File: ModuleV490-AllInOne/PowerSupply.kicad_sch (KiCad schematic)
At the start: 28 parts, among them J5 POWER_IN, J9 BYPASS, U10 XL7005A, U11 AP2204K-5.0TRG1, U12 XC6206-1.8NR, U9 XC6206-3.3V

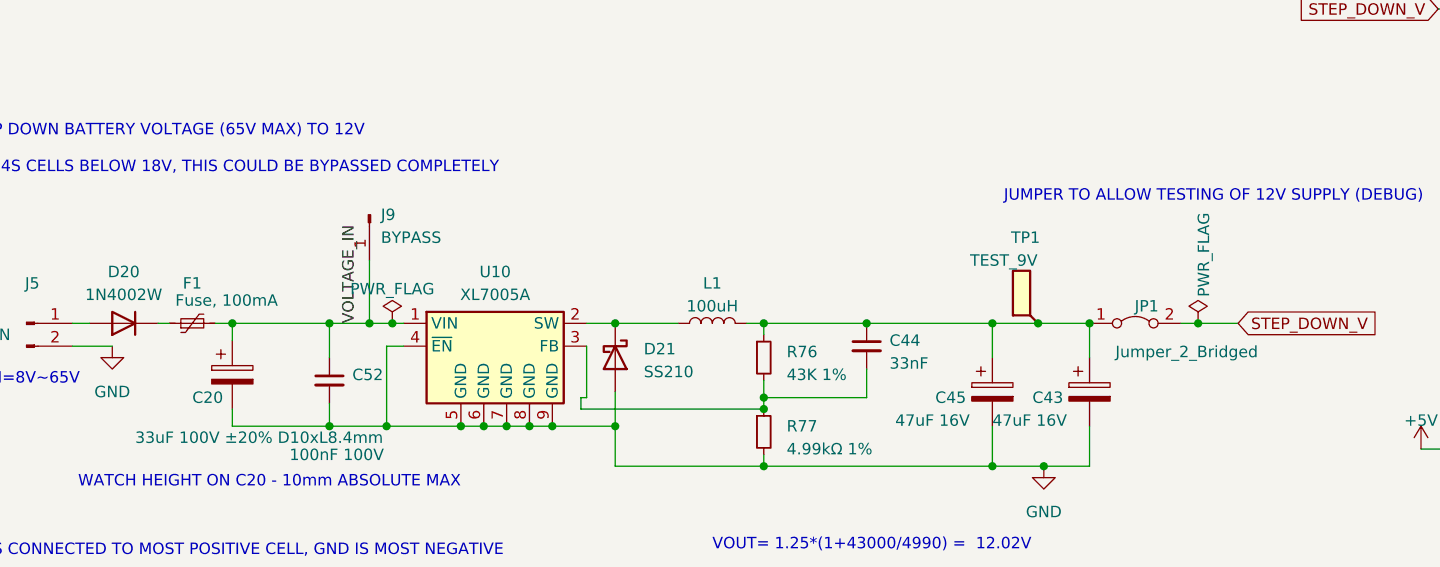
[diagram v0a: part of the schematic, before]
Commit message: Squashed commit of the following:
commit 382df4b7a104fb34cc4a4da3f786b21ade19fcd5
Author: GitHub Action <action@github.com>
Date:   Fri Apr 18 11:47:05 2025 +0000

    CI: pcb-artifacts-ModuleV490-AllInOne

commit b35cb7a0d3894cf57b33edb037eb829bc9ec5ea4
Author: Stuart Pittaway <1201909+stuartpittaway@users.noreply.github.com>
Date:   Fri Apr 18 12:44:57 2025 +0100

    Minor tweaks

commit ea046b7e5d836263693da1b47c6dfb3dc918925c
Author: Stuart Pittaway <1201909+stuartpittaway@users.noreply.github.com>
Date:   Fri Apr 18 12:44:16 2025 +0100

    PCB Panel of Temp sensors

commit ba929f4700586b6858203bc466c6b18e911d661e
Author: GitHub Action <action@github.com>
Date:   Sun Mar 23 15:29:50 2025 +0000

    CI: pcb-artifacts-ModuleV490-AllInOne

commit 1dbbac7378fdc5acb48c43d3f728917ce2318f16
Author: GitHub Action <action@github.com>
Date:   Wed Apr 10 09:57:21 2024 +0000

    CI: pcb-artifacts-ModuleV490-AllInOne

commit 35f617d42fc7a6a7ab395d232005d3307c26595c
Author: Stuart Pittaway <1201909+stuartpittaway@users.noreply.github.com>
Date:   Wed Apr 10 10:55:49 2024 +0100

    Update pcb-artifacts-modulev490-allinone.yaml

commit c8295c0089ea2c5e86742be6a5572142963deb8f
Author: Stuart Pittaway <1201909+stuartpittaway@users.noreply.github.com>
Date:   Wed Apr 10 10:53:50 2024 +0100

    Update pcb-artifacts-modulev490-allinone.yaml

commit d19b2989a6afd4cac4ecf3c8c78554eedba7b99a
Author: Stuart Pittaway <1201909+stuartpittaway@users.noreply.github.com>
Date:   Wed Apr 10 10:50:28 2024 +0100

    Update pcb-artifacts-modulev490-allinone.yaml

commit 8478886fe70d1ee53aca3bbd908099e6f38ff11d
Author: Stuart Pittaway <1201909+stuartpittaway@users.noreply.github.com>
Date:   Wed Apr 10 10:41:28 2024 +0100

    Update pcb-artifacts-modulev490-allinone.yaml

commit afeafa74721a9b51459c6106f0a15ae423229204
Author: Stuart Pittaway <1201909+stuartpittaway@users.noreply.github.com>
Date:   Wed Apr 10 10:39:10 2024 +0100

    Inductor part change - fix workflows

commit 70fd25ba43b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
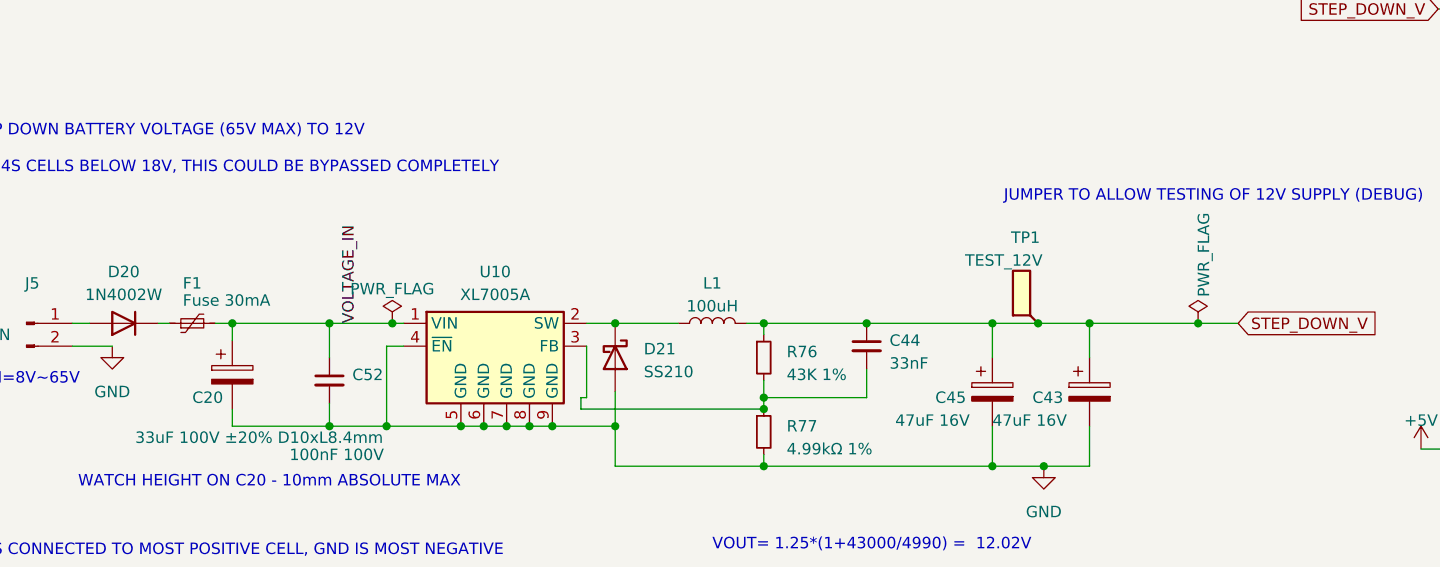
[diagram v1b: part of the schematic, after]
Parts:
- removed J9: BYPASS, Connector_PinSocket_2.54mm:PinSocket_1x01_P2.54mm_Vertical, symbol Connector:Conn_01x01_Pin
- removed JP1: Jumper_2_Bridged, Connector_PinHeader_2.54mm:PinHeader_1x02_P2.54mm_Vertical, symbol Jumper:Jumper_2_Bridged
- F1: value Fuse, 100mA -> Fuse 30mA; footprint Fuse:Fuse_Bourns_MF-RHT100 -> Fuse:Fuse_0805_2012Metric; LCSCStockCode C2680606 -> C19273358; PartNumber JK250-100U -> 0805L003/80XR
- L1: footprint COILMX:MS1040-101M -> Inductor_SMD:L_1008_2520Metric_Pad1.43x2.20mm_HandSolder; LCSCStockCode C380060 -> C286551; PartNumber MS1040-101M -> NLV25T-101J-EF
- TP1: value TEST_9V -> TEST_12V
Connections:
- net STEP_DOWN_V: now also C43.1, C44.1, C45.1, L1.2, R76.1, TP1.1
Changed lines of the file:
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@@
   (junction (at 228.6 121.285) (diameter 0) (color 0 0 0 0)
   )
+  (junction (at 210.185 48.26) (diameter 0) (color 0 0 0 0)
+  )
+  (junction (at 64.135 73.025) (diameter 0) (color 0 0 0 0)
+  )
+  (junction (at 208.28 131.445) (diameter 0) (color 0 0 0 0)
+  )
+  (junction (at 64.135 84.455) (diameter 0) (color 0 0 0 0)
+  )
+  (junction (at 205.105 97.155) (diameter 0) (color 0 0 0 0)
+  )
+  (junction (at 112.395 81.28) (diameter 0) (color 0 0 0 0)
+  )
+  (junction (at 70.485 84.455) (diameter 0) (color 0 0 0 0)
+  )
+  (junction (at 78.74 84.455) (diameter 0) (color 0 0 0 0)
+  )
+  (junction (at 201.295 38.1) (diameter 0) (color 0 0 0 0)
+  )
+  (junction (at 88.9 84.455) (diameter 0) (color 0 0 0 0)
+  )
+  (junction (at 191.135 121.285) (diameter 0) (color 0 0 0 0)
+  )
+  (junction (at 219.71 121.285) (diameter 0) (color 0 0 0 0)
+  )
+  (junction (at 71.12 73.025) (diameter 0) (color 0 0 0 0)
+  )
+  (junction (at 53.34 73.025) (diameter 0) (color 0 0 0 0)
+  )
+  (junction (at 143.51 88.9) (diameter 0) (color 0 0 0 0)
+  )
+  (junction (at 137.795 88.9) (diameter 0) (color 0 0 0 0)
+  )
+  (junction (at 112.395 88.9) (diameter 0) (color 0 0 0 0)
+  )
+  (junction (at 123.825 73.025) (diameter 0) (color 0 0 0 0)
+  )
+  (junction (at 228.6 86.995) (diameter 0) (color 0 0 0 0)
+  )
+  (junction (at 142.875 73.025) (diameter 0) (color 0 0 0 0)
+  )
+  (junction (at 95.885 73.025) (diameter 0) (color 0 0 0 0)
+  )
   (junction (at 148.59 73.025) (diameter 0) (color 0 0 0 0)
   )
-  (junction (at 210.185 48.26) (diameter 0) (color 0 0 0 0)
-  )
-  (junction (at 64.135 73.025) (diameter 0) (color 0 0 0 0)
-  )
-  (junction (at 208.28 131.445) (diameter 0) (color 0 0 0 0)
-  )
-  (junction (at 64.135 84.455) (diameter 0) (color 0 0 0 0)
-  )
-  (junction (at 205.105 97.155) (diameter 0) (color 0 0 0 0)
-  )
-  (junction (at 112.395 81.28) (diameter 0) (color 0 0 0 0)
-  )
-  (junction (at 70.485 84.455) (diameter 0) (color 0 0 0 0)
-  )
-  (junction (at 78.74 84.455) (diameter 0) (color 0 0 0 0)
-  )
-  (junction (at 201.295 38.1) (diameter 0) (color 0 0 0 0)
-  )
-  (junction (at 88.9 84.455) (diameter 0) (color 0 0 0 0)
-  )
-  (junction (at 191.135 121.285) (diameter 0) (color 0 0 0 0)
-  )
-  (junction (at 219.71 121.285) (diameter 0) (color 0 0 0 0)
-  )
-  (junction (at 71.12 73.025) (diameter 0) (color 0 0 0 0)
-  )
-  (junction (at 68.58 73.025) (diameter 0) (color 0 0 0 0)
-  )
-  (junction (at 53.34 73.025) (diameter 0) (color 0 0 0 0)
-  )
-  (junction (at 143.51 88.9) (diameter 0) (color 0 0 0 0)
-  )
-  (junction (at 137.795 88.9) (diameter 0) (color 0 0 0 0)
-  )
-  (junction (at 112.395 88.9) (diameter 0) (color 0 0 0 0)
-  )
-  (junction (at 123.825 73.025) (diameter 0) (color 0 0 0 0)
-  )
-  (junction (at 228.6 86.995) (diameter 0) (color 0 0 0 0)
-  )
-  (junction (at 142.875 73.025) (diameter 0) (color 0 0 0 0)
-  )
-  (junction (at 95.885 73.025) (diameter 0) (color 0 0 0 0)
-  )
   (junction (at 137.795 73.025) (diameter 0) (color 0 0 0 0)
   )
+  (junction (at 160.655 73.025) (diameter 0) (color 0 0 0 0)
+  )
   (junction (at 221.615 38.1) (diameter 0) (color 0 0 0 0)
   )
@@
   (junction (at 112.395 73.025) (diameter 0) (color 0 0 0 0)
   )
-  (junction (at 160.655 73.025) (diameter 0) (color 0 0 0 0)
-  )
   (junction (at 219.71 86.995) (diameter 0) (color 0 0 0 0)
   )
@@
     (stroke (width 0) (type default))
   )
-  (wire (pts (xy 68.58 73.025) (xy 71.12 73.025))
-    (stroke (width 0) (type default))
-  )
   (wire (pts (xy 53.34 84.455) (xy 64.135 84.455))
     (stroke (width 0) (type default))
@@
     (stroke (width 0) (type default))
   )
-  (wire (pts (xy 158.75 73.025) (xy 160.655 73.025))
-    (stroke (width 0) (type default))
-  )
   (wire (pts (xy 207.01 48.26) (xy 210.185 48.26))
     (stroke (width 0) (type default))
@@
     (stroke (width 0) (type default))
   )
-  (wire (pts (xy 68.58 66.04) (xy 68.58 73.025))
-    (stroke (width 0) (type default))
-  )
   (wire (pts (xy 70.485 75.565) (xy 70.485 84.455))
     (stroke (width 0) (type default))
@@
     (stroke (width 0) (type default))
   )
-  (wire (pts (xy 64.135 73.025) (xy 68.58 73.025))
+  (wire (pts (xy 64.135 73.025) (xy 71.12 73.025))
     (stroke (width 0) (type default))
   )
@@
   )
   (wire (pts (xy 53.34 73.025) (xy 64.135 73.025))
+    (stroke (width 0) (type default))
+  )
+  (wire (pts (xy 148.59 73.025) (xy 160.655 73.025))
     (stroke (width 0) (type default))
   )
@@
         (path "/e63e39d7-6ac0-4ffd-8aa3-1841a4541b55/8dad0a00-271a-4077-b7a7-daab5ad043ac"
           (reference "C52") (unit 1)
-        )
-      )
-    )
-  )
-  (symbol (lib_id "Jumper:Jumper_2_Bridged") (at 153.67 73.025 0) (unit 1)
-    (in_bom yes) (on_board yes) (dnp no)
-    (property "Reference" "JP1" (at 154.94 71.12 0)
-      (effects (font (size 1.27 1.27)))
-    )
-    (property "Value" "Jumper_2_Bridged" (at 159.385 76.2 0)
-      (effects (font (size 1.27 1.27)))
-    )
-    (property "Footprint" "Connector_PinHeader_2.54mm:PinHeader_1x02_P2.54mm_Vertical" (at 153.67 73.025 0)
-      (effects (font (size 1.27 1.27)) hide)
-    )
-    (property "Datasheet" "~" (at 153.67 73.025 0)
-      (effects (font (size 1.27 1.27)) hide)
-    )
-    (property "PartNumber" "DZ254R-11-02-63" (at 153.67 73.025 0)
-      (effects (font (size 1.27 1.27)) hide)
-    )
-    (property "LCSCStockCode" "C2935908" (at 153.67 73.025 0)
-      (effects (font (size 1.27 1.27)) hide)
-    )
-    (pin "1")
-    (pin "2")
-    (instances
-      (project "Module_16S"
-        (path "/e63e39d7-6ac0-4ffd-8aa3-1841a4541b55/8dad0a00-271a-4077-b7a7-daab5ad043ac"
-          (reference "JP1") (unit 1)
         )
       )
@@
     )
   )
-  (symbol (lib_id "Connector:Conn_01x01_Pin") (at 68.58 60.96 270) (unit 1)
-    (in_bom no) (on_board yes) (dnp no) (fields_autoplaced)
-    (property "Reference" "J9" (at 69.85 60.96 90)
-      (effects (font (size 1.27 1.27)) (justify left))
-    )
-    (property "Value" "BYPASS" (at 69.85 63.5 90)
-      (effects (font (size 1.27 1.27)) (justify left))
-    )
-    (property "Footprint" "Connector_PinSocket_2.54mm:PinSocket_1x01_P2.54mm_Vertical" (at 68.58 60.96 0)
-      (effects (font (size 1.27 1.27)) hide)
-    )
-    (property "Datasheet" "~" (at 68.58 60.96 0)
-      (effects (font (size 1.27 1.27)) hide)
-    )
-    (pin "1")
-    (instances
-      (project "Module_16S"
-        (path "/e63e39d7-6ac0-4ffd-8aa3-1841a4541b55/8dad0a00-271a-4077-b7a7-daab5ad043ac"
-          (reference "J9") (unit 1)
-        )
-      )
-    )
-  )
   (symbol (lib_id "power:GND") (at 40.005 75.565 0) (unit 1)
     (in_bom yes) (on_board yes) (dnp no) (fields_autoplaced)
@@
       (effects (font (size 1.27 1.27)))
     )
-    (property "Footprint" "COILMX:MS1040-101M" (at 106.68 73.025 0)
+    (property "Footprint" "Inductor_SMD:L_1008_2520Metric_Pad1.43x2.20mm_HandSolder" (at 106.68 73.025 0)
       (effects (font (size 1.27 1.27)) hide)
     )
@@
       (effects (font (size 1.27 1.27)) hide)
     )
-    (property "PartNumber" "MS1040-101M" (at 106.68 73.025 0)
-      (effects (font (size 1.27 1.27)) hide)
-    )
-    (property "LCSCStockCode" "C380060" (at 106.68 73.025 0)
+    (property "PartNumber" "NLV25T-101J-EF" (at 106.68 73.025 0)
+      (effects (font (size 1.27 1.27)) hide)
+    )
+    (property "LCSCStockCode" "C286551" (at 106.68 73.025 0)
       (effects (font (size 1.27 1.27)) hide)
     )
@@
       (effects (font (size 1.27 1.27)))
     )
-    (property "Value" "Fuse, 100mA" (at 52.705 70.485 90)
-      (effects (font (size 1.27 1.27)))
-    )
-    (property "Footprint" "Fuse:Fuse_Bourns_MF-RHT100" (at 53.975 71.755 0)
+    (property "Value" "Fuse 30mA" (at 52.705 70.485 90)
+      (effects (font (size 1.27 1.27)))
+    )
+    (property "Footprint" "Fuse:Fuse_0805_2012Metric" (at 53.975 71.755 0)
       (effects (font (size 1.27 1.27)) (justify left) hide)
     )
-    (property "Datasheet" "https://datasheet.lcsc.com/lcsc/2304140030_Jinrui-Electronic-Materials-Co--JK250-100U_C2680606.pdf" (at 48.895 73.025 0)
-      (effects (font (size 1.27 1.27)) hide)
-    )
-    (property "PartNumber" "JK250-100U" (at 48.895 73.025 90)
-      (effects (font (size 1.27 1.27)) hide)
-    )
-    (property "LCSCStockCode" "C2680606" (at 48.895 73.025 0)
+    (property "Datasheet" "https://wmsc.lcsc.com/wmsc/upload/file/pdf/v2/lcsc/2312012005_LUTE-0805L003-80XR_C19273358.pdf" (at 48.895 73.025 0)
+      (effects (font (size 1.27 1.27)) hide)
+    )
+    (property "PartNumber" "0805L003/80XR" (at 48.895 73.025 90)
+      (effects (font (size 1.27 1.27)) hide)
+    )
+    (property "LCSCStockCode" "C19273358" (at 48.895 73.025 0)
       (effects (font (size 1.27 1.27)) hide)
     )
@@
       (effects (font (size 1.27 1.27)))
     )
-    (property "Value" "TEST_9V" (at 139.065 66.04 90)
-      (effects (font (size 1.27 1.27)))
-    )
+    (property "Value" "TEST_12V" (at 139.065 66.04 90)
+      (effects (font (size 1.27 1.27)))
+    )
